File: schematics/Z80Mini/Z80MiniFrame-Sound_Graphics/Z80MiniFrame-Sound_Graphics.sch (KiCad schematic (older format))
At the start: 3 parts, among them J1 Conn_02x20_Odd_Even, U13 74LS139

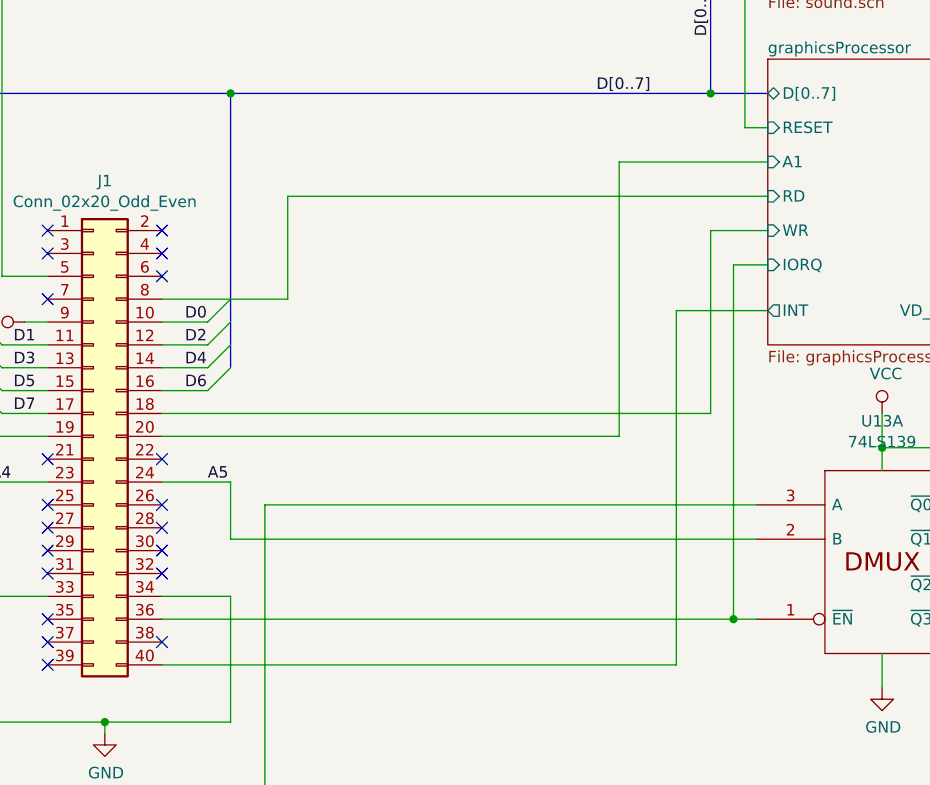
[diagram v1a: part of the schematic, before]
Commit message: Latest modifications
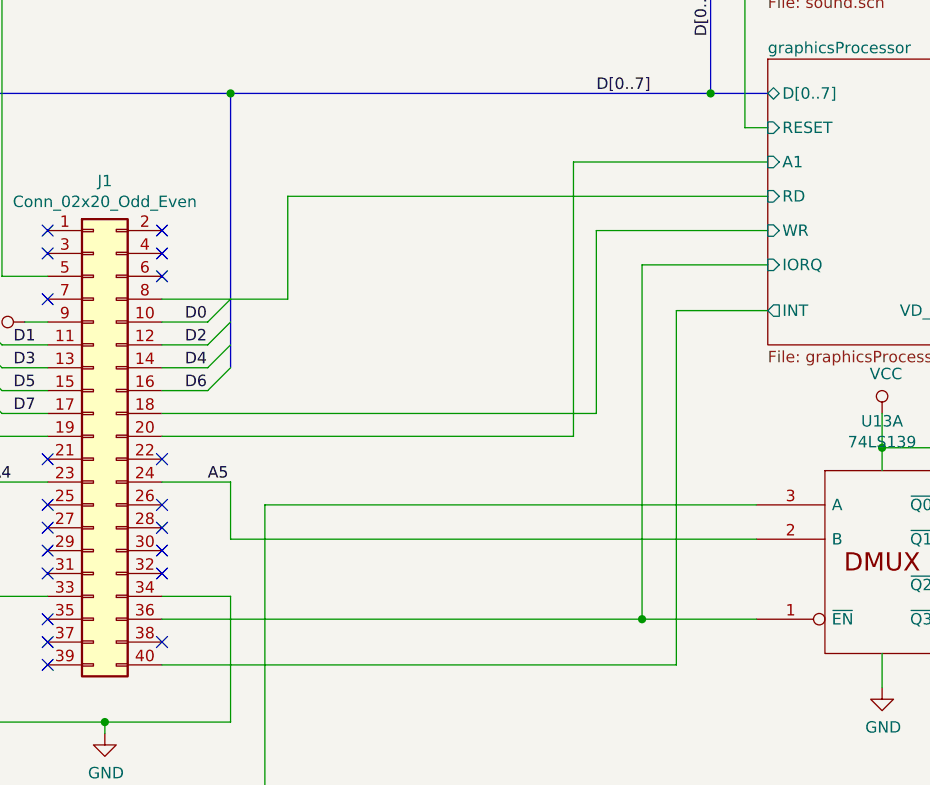
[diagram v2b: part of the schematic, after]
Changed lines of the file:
@@
 	4950 2600 1700 2600
 Wire Wire Line
-	2400 5300 4400 5300
+	2400 5300 4200 5300
 Wire Wire Line
-	4400 5300 4400 4100
+	4200 5300 4200 4100
 Wire Wire Line
-	4400 4100 5050 4100
+	2400 6100 4500 6100
 Wire Wire Line
-	2400 6100 4900 6100
-Wire Wire Line
-	4900 6100 4900 4550
-Wire Wire Line
-	4900 4550 5050 4550
+	4500 6100 4500 4550
 Wire Wire Line
 	5050 4250 2950 4250
 Wire Wire Line
 	2950 4250 2950 4700
-Wire Wire Line
-	2400 5200 4800 5200
-Wire Wire Line
-	4800 5200 4800 4400
-Wire Wire Line
-	4800 4400 5050 4400
 $Comp
 L 74xx_IEEE:74LS139 U13
@@
 Wire Wire Line
 	6600 4750 5950 4750
-Wire Wire Line
-	5000 6100 4900 6100
-Connection ~ 4900 6100
 Wire Wire Line
 	5000 5750 2700 5750
@@
 NoConn ~ 1900 6300
 Wire Wire Line
+	4300 5200 4300 4400
+Wire Wire Line
+	2400 5200 4300 5200
+Wire Wire Line
+	4300 4400 5050 4400
+Connection ~ 4500 6100
+Wire Wire Line
+	4500 6100 5000 6100
+Wire Wire Line
+	4500 4550 5050 4550
+Wire Wire Line
+	4200 4100 5050 4100
+Wire Wire Line
 	2400 4700 2950 4700
